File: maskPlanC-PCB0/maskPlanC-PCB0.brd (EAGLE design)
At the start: 25 x 20 mm, 8 parts, among them U1 ATTINY85-20PU

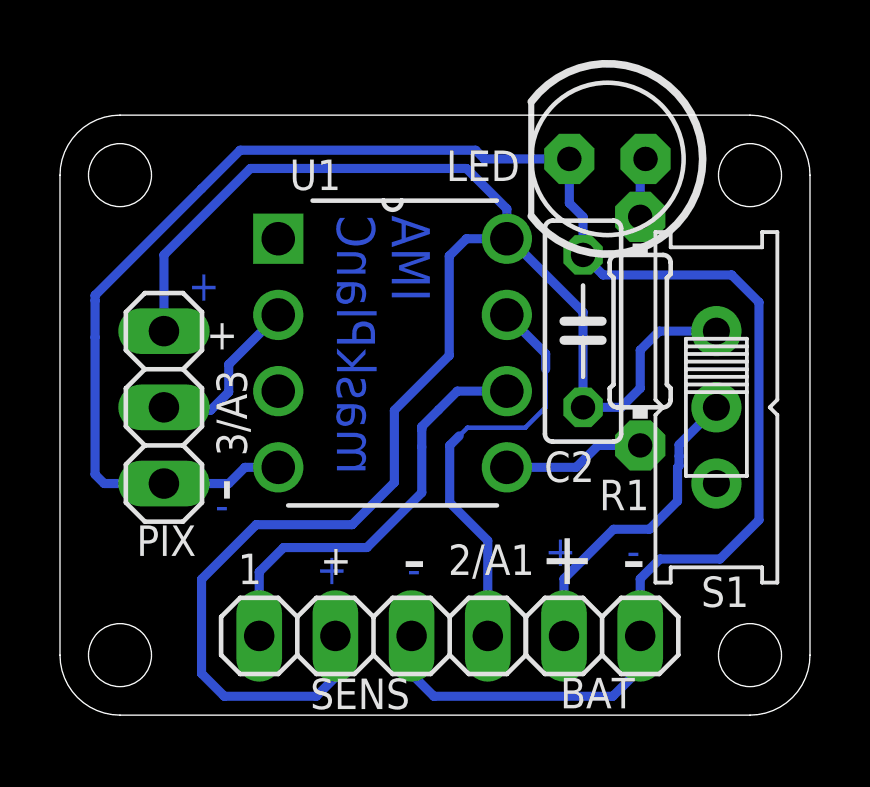
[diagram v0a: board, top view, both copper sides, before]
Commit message: CAM v1
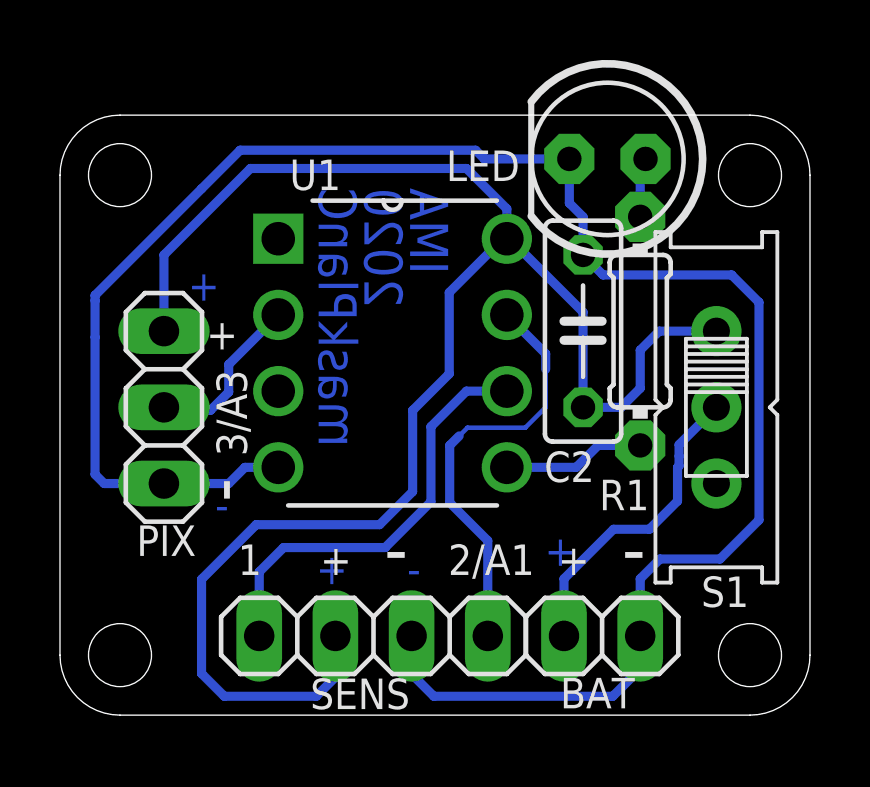
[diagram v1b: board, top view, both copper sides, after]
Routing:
- net N$7: track 14.7 -> 14.2 mm
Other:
- board text added: "2020"
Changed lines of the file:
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@@
 <wire x1="34" y1="56" x2="34" y2="40" width="0" layer="20"/>
 <wire x1="34" y1="40" x2="36" y2="38" width="0" layer="20" curve="90"/>
-<text x="44.5008" y="54.6608" size="1.27" layer="16" font="vector" ratio="15" rot="MR270">maskPlanC</text>
+<text x="43.8912" y="55.5752" size="1.27" layer="16" font="vector" ratio="15" rot="MR270">maskPlanC</text>
 <hole x="36" y="40" drill="2.1"/>
 <hole x="57" y="40" drill="2.1"/>
@@
 <text x="53.34" y="42.9768" size="1.016" layer="16" rot="MR0">-</text>
 <text x="40.2336" y="45.1104" size="1.778" layer="25" rot="R90">-</text>
-<text x="45.4152" y="42.3672" size="1.778" layer="25">-</text>
-<text x="52.7304" y="42.3672" size="1.778" layer="25">-</text>
+<text x="44.8056" y="42.672" size="1.778" layer="25">-</text>
+<text x="52.7304" y="42.672" size="1.778" layer="25">-</text>
 <text x="39.9288" y="51.2064" size="1.016" layer="25" rot="R180">+</text>
 <text x="42.672" y="42.672" size="1.016" layer="25">+</text>
-<text x="49.9872" y="42.3672" size="1.778" layer="25">+</text>
+<text x="50.5968" y="42.672" size="1.016" layer="25">+</text>
 <text x="40.2336" y="46.6344" size="1.016" layer="25" rot="R90">3/A3</text>
 <text x="46.9392" y="42.672" size="1.016" layer="25">2/A1</text>
-<text x="39.9288" y="42.3672" size="1.016" layer="25">1</text>
-<text x="46.3296" y="54.6608" size="1.27" layer="16" font="vector" ratio="15" rot="MR270">IMA</text>
+<text x="39.9288" y="42.672" size="1.016" layer="25">1</text>
+<text x="45.4152" y="55.5752" size="1.27" layer="16" font="vector" ratio="15" rot="MR270">2020</text>
+<text x="46.9392" y="55.5752" size="1.27" layer="16" font="vector" ratio="15" rot="MR270">IMA</text>
 </plain>
 <attributes>
@@
 <wire x1="52.705" y1="48.26" x2="53.34" y2="48.895" width="0.3048" layer="16"/>
 <wire x1="40.347" y1="56.222" x2="47.5488" y2="56.222" width="0.3048" layer="16"/>
-<wire x1="47.5488" y1="53.88" x2="48.895" y2="53.88" width="0.3048" layer="16"/>
-<wire x1="46.974" y1="53.3052" x2="47.5488" y2="53.88" width="0.3048" layer="16"/>
+<wire x1="48.768" y1="53.88" x2="48.895" y2="53.88" width="0.3048" layer="16"/>
+<wire x1="46.974" y1="52.086" x2="48.768" y2="53.88" width="0.3048" layer="16"/>
 <wire x1="48.895" y1="54.8758" x2="47.5488" y2="56.222" width="0.3048" layer="16"/>
 <wire x1="48.895" y1="53.88" x2="48.895" y2="54.8758" width="0.3048" layer="16"/>
-<wire x1="45.1452" y1="48.1584" x2="45.1452" y2="45.7548" width="0.3048" layer="16"/>
-<wire x1="43.7388" y1="44.3484" x2="45.1452" y2="45.7548" width="0.3048" layer="16"/>
-<wire x1="40.5384" y1="44.3484" x2="43.7388" y2="44.3484" width="0.3048" layer="16"/>
+<wire x1="45.7548" y1="48.1584" x2="45.7548" y2="45.45" width="0.3048" layer="16"/>
+<wire x1="44.6532" y1="44.3484" x2="45.7548" y2="45.45" width="0.3048" layer="16"/>
+<wire x1="40.5384" y1="44.3484" x2="44.6532" y2="44.3484" width="0.3048" layer="16"/>
 <wire x1="38.7184" y1="42.5284" x2="40.5384" y2="44.3484" width="0.3048" layer="16"/>
 <wire x1="37.465" y1="50.8" x2="37.465" y2="53.34" width="0.3048" layer="16"/>
 <wire x1="37.465" y1="53.34" x2="40.347" y2="56.222" width="0.3048" layer="16"/>
-<wire x1="45.1452" y1="48.1584" x2="46.974" y2="49.9872" width="0.3048" layer="16"/>
-<wire x1="46.974" y1="49.9872" x2="46.974" y2="53.3052" width="0.3048" layer="16"/>
+<wire x1="45.7548" y1="48.1584" x2="46.974" y2="49.3776" width="0.3048" layer="16"/>
+<wire x1="46.974" y1="49.3776" x2="46.974" y2="52.086" width="0.3048" layer="16"/>
 </signal>
 <signal name="N$3">
@@
 <contactref element="U1" pad="6"/>
 <contactref element="SENS" pad="1"/>
-<wire x1="48.895" y1="48.8" x2="47.244" y2="48.8" width="0.3048" layer="16"/>
-<wire x1="46.6184" y1="48.1744" x2="47.244" y2="48.8" width="0.3048" layer="16"/>
+<wire x1="48.895" y1="48.8" x2="47.5488" y2="48.8" width="0.3048" layer="16"/>
 <wire x1="40.64" y1="40.64" x2="40.64" y2="42.7736" width="0.3048" layer="16"/>
 <wire x1="40.64" y1="42.7736" x2="41.4528" y2="43.5864" width="0.3048" layer="16"/>
-<wire x1="41.4528" y1="43.5864" x2="44.2308" y2="43.5864" width="0.3048" layer="16"/>
-<wire x1="44.2308" y1="43.5864" x2="46.0596" y2="45.4152" width="0.3048" layer="16"/>
-<wire x1="46.0596" y1="45.4152" x2="46.0596" y2="46.9392" width="0.3048" layer="16"/>
-<wire x1="46.0596" y1="46.9392" x2="46.0596" y2="47.514" width="0.3048" layer="16"/>
-<wire x1="46.0596" y1="47.514" x2="46.0596" y2="47.6156" width="0.3048" layer="16"/>
-<wire x1="46.0596" y1="47.6156" x2="46.6184" y2="48.1744" width="0.3048" layer="16"/>
+<wire x1="41.4528" y1="43.5864" x2="44.8404" y2="43.5864" width="0.3048" layer="16"/>
+<wire x1="44.8404" y1="43.5864" x2="46.3644" y2="45.1104" width="0.3048" layer="16"/>
+<wire x1="46.3644" y1="45.1104" x2="46.3644" y2="47.6156" width="0.3048" layer="16"/>
+<wire x1="46.3644" y1="47.6156" x2="47.5488" y2="48.8" width="0.3048" layer="16"/>
 </signal>
 <signal name="N$7">
@@
 <wire x1="47.3075" y1="47.3075" x2="47.5808" y2="47.5808" width="0.1524" layer="16"/>
 <wire x1="47.5808" y1="47.5808" x2="49.507775" y2="47.5808" width="0.1524" layer="16"/>
-<wire x1="50.1904" y1="48.263425" x2="50.1904" y2="48.895" width="0.1524" layer="16"/>
-<wire x1="50.1904" y1="48.895" x2="50.1904" y2="49.53" width="0.1524" layer="16"/>
-<wire x1="50.1904" y1="49.53" x2="50.1904" y2="50.0446" width="0.1524" layer="16"/>
+<wire x1="50.1904" y1="48.263425" x2="50.1904" y2="49.53" width="0.1524" layer="16"/>
 </signal>
 </signals>
